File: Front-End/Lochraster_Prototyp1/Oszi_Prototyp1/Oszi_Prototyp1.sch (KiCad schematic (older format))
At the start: 9 parts, among them IC1 LTC1420CGN#PBF, J1 FPGA_GPIO, J2 input

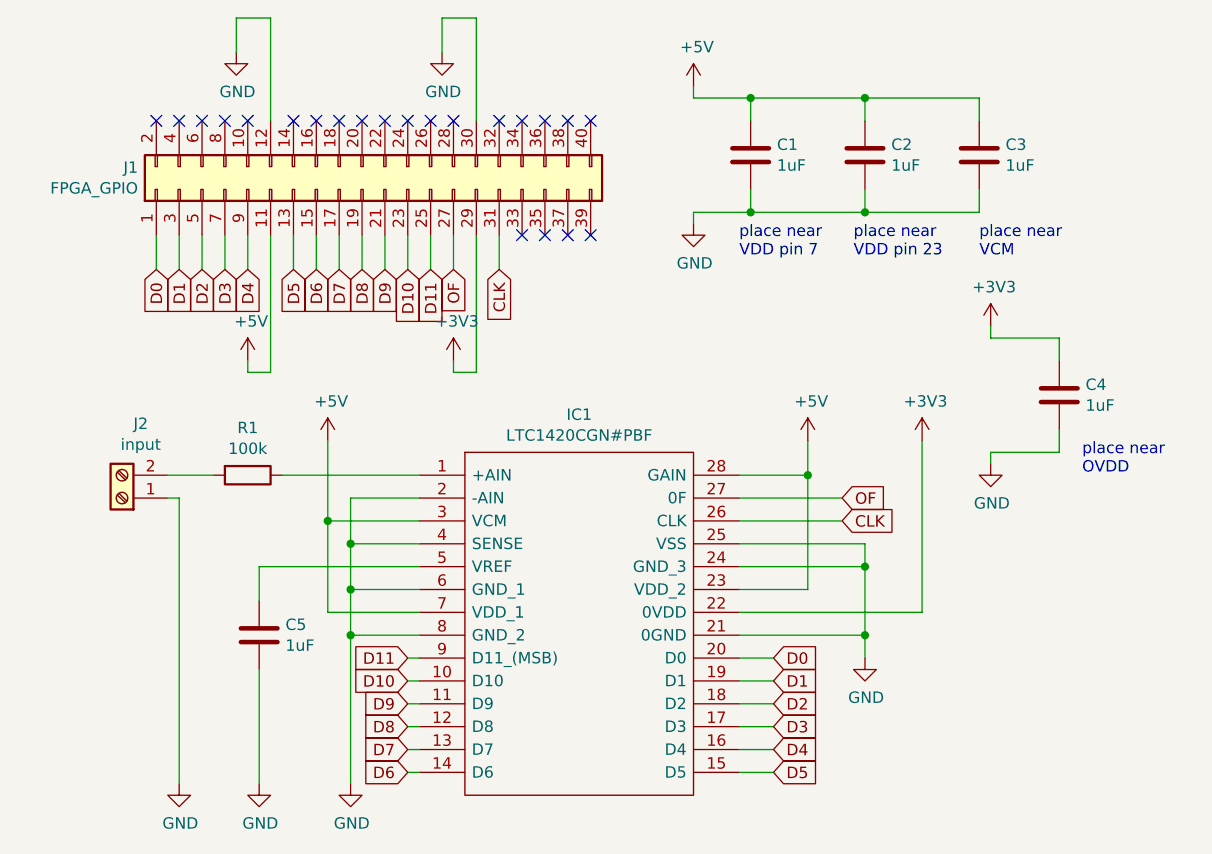
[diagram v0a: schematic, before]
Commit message: 18.03.202123:41:19,54
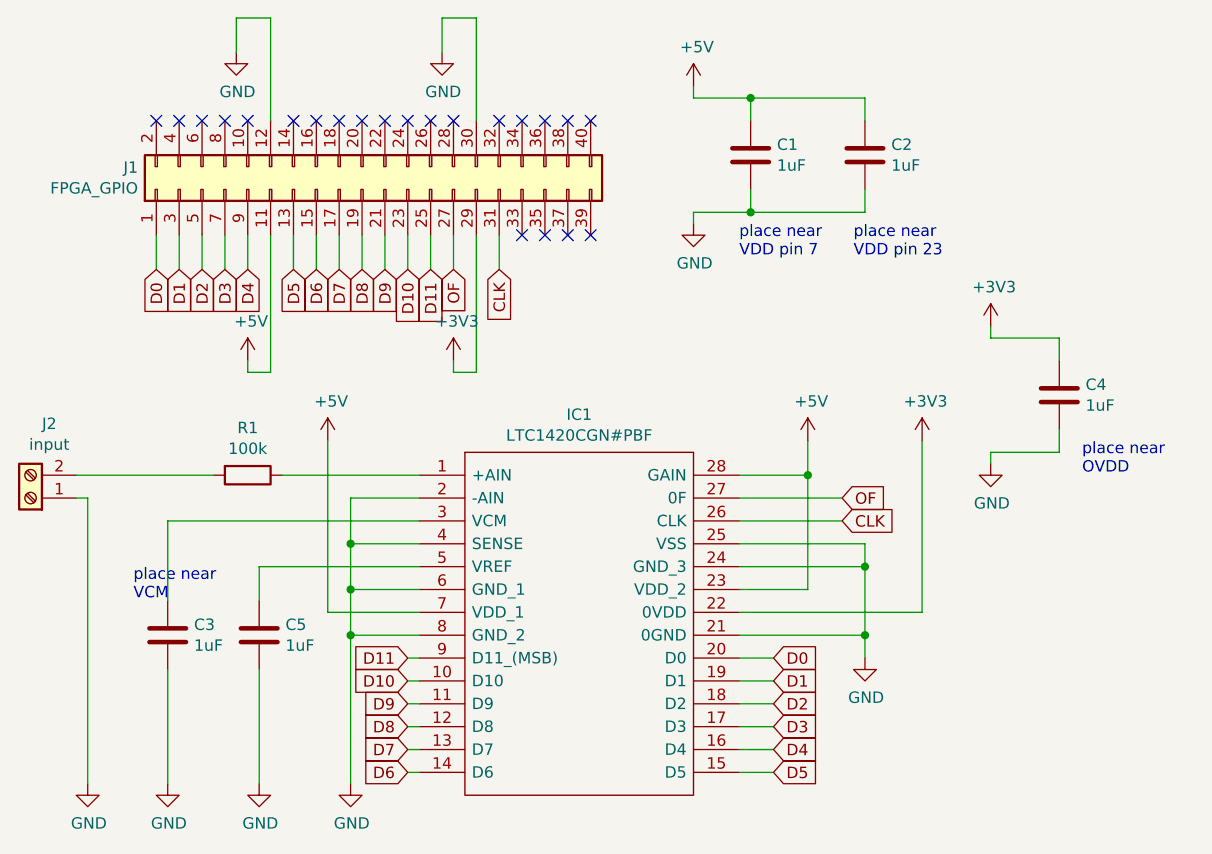
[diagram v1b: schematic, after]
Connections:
- net +5V: no longer C3.1, IC1.3 (VCM)
- new net: C3.1, IC1.3 (VCM)
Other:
- moved on the sheet: C3, J2
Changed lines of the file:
@@
 L Device:C C3
 U 1 1 604A41B4
-P 9100 1200
-F 0 "C3" H 9215 1246 50  0000 L CNN
-F 1 "1uF" H 9215 1155 50  0000 L CNN
-F 2 "Capacitor_SMD:C_1206_3216Metric_Pad1.42x1.75mm_HandSolder" H 9138 1050 50  0001 C CNN
-F 3 "~" H 9100 1200 50  0001 C CNN
-	1    9100 1200
+P 5550 3300
+F 0 "C3" H 5665 3346 50  0000 L CNN
+F 1 "1uF" H 5665 3255 50  0000 L CNN
+F 2 "Capacitor_SMD:C_1206_3216Metric_Pad1.42x1.75mm_HandSolder" H 5588 3150 50  0001 C CNN
+F 3 "~" H 5550 3300 50  0001 C CNN
+	1    5550 3300
 	1    0    0    -1
 $EndComp
@@
 	7850 950  8100 950
 Wire Wire Line
-	9100 1050 9100 950
-Wire Wire Line
 	8600 1050 8600 950
-Connection ~ 8600 950
-Wire Wire Line
-	8600 950  9100 950
 Wire Wire Line
 	8100 1050 8100 950
@@
 	7850 1450 8100 1450
 Wire Wire Line
-	9100 1350 9100 1450
-Wire Wire Line
 	8600 1350 8600 1450
-Connection ~ 8600 1450
-Wire Wire Line
-	8600 1450 9100 1450
 Wire Wire Line
 	8100 1350 8100 1450
@@
 Wire Wire Line
 	6650 3200 6250 3200
-Wire Wire Line
-	6250 3200 6250 2800
-Wire Wire Line
-	6650 2800 6250 2800
-Connection ~ 6250 2800
-Wire Wire Line
-	6250 2800 6250 2450
 $Comp
 L power:GND #PWR0111
@@
 Wire Wire Line
 	5950 3950 5950 3450
-Text Notes 9100 1650 0    50   ~ 0
+Text Notes 5400 3150 0    50   ~ 0
 place near\nVCM\n
 Wire Wire Line
@@
 L Connector:Screw_Terminal_01x02 J2
 U 1 1 604C527E
-P 5350 2700
-F 0 "J2" H 5268 2375 50  0000 C CNN
-F 1 "input" H 5268 2466 50  0000 C CNN
-F 2 "Connector_PinSocket_2.54mm:PinSocket_1x02_P2.54mm_Horizontal" H 5350 2700 50  0001 C CNN
-F 3 "~" H 5350 2700 50  0001 C CNN
-	1    5350 2700
+P 4950 2700
+F 0 "J2" H 4868 2375 50  0000 C CNN
+F 1 "input" H 4868 2466 50  0000 C CNN
+F 2 "Connector_PinSocket_2.54mm:PinSocket_1x02_P2.54mm_Horizontal" H 4950 2700 50  0001 C CNN
+F 3 "~" H 4950 2700 50  0001 C CNN
+	1    4950 2700
 	-1   0    0    1
 $EndComp
@@
 Wire Wire Line
 	6650 2600 6050 2600
-Wire Wire Line
-	5750 2600 5550 2600
 $Comp
 L power:GND #PWR0113
 U 1 1 604CA2F6
-P 5600 3950
-F 0 "#PWR0113" H 5600 3700 50  0001 C CNN
-F 1 "GND" H 5605 3777 50  0000 C CNN
-F 2 "" H 5600 3950 50  0001 C CNN
-F 3 "" H 5600 3950 50  0001 C CNN
-	1    5600 3950
-	1    0    0    -1
-$EndComp
-Wire Wire Line
-	5600 3950 5600 2700
-Wire Wire Line
-	5600 2700 5550 2700
+P 5200 3950
+F 0 "#PWR0113" H 5200 3700 50  0001 C CNN
+F 1 "GND" H 5205 3777 50  0000 C CNN
+F 2 "" H 5200 3950 50  0001 C CNN
+F 3 "" H 5200 3950 50  0001 C CNN
+	1    5200 3950
+	1    0    0    -1
+$EndComp
+Wire Wire Line
+	5200 3950 5200 2700
+Wire Wire Line
+	5200 2700 5150 2700
 $Comp
 L power:GND #PWR0114
@@
 NoConn ~ 7200 1550
 NoConn ~ 7100 1550
+Wire Wire Line
+	6250 2450 6250 3200
+Wire Wire Line
+	6650 2800 5550 2800
+Wire Wire Line
+	5550 2800 5550 3150
+$Comp
+L power:GND #PWR?
+U 1 1 6054611D
+P 5550 3950
+F 0 "#PWR?" H 5550 3700 50  0001 C CNN
+F 1 "GND" H 5555 3777 50  0000 C CNN
+F 2 "" H 5550 3950 50  0001 C CNN
+F 3 "" H 5550 3950 50  0001 C CNN
+	1    5550 3950
+	1    0    0    -1
+$EndComp
+Wire Wire Line
+	5550 3950 5550 3450
+Wire Wire Line
+	5150 2600 5750 2600
 $EndSCHEMATC
